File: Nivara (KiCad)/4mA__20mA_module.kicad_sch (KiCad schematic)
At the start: 2 parts

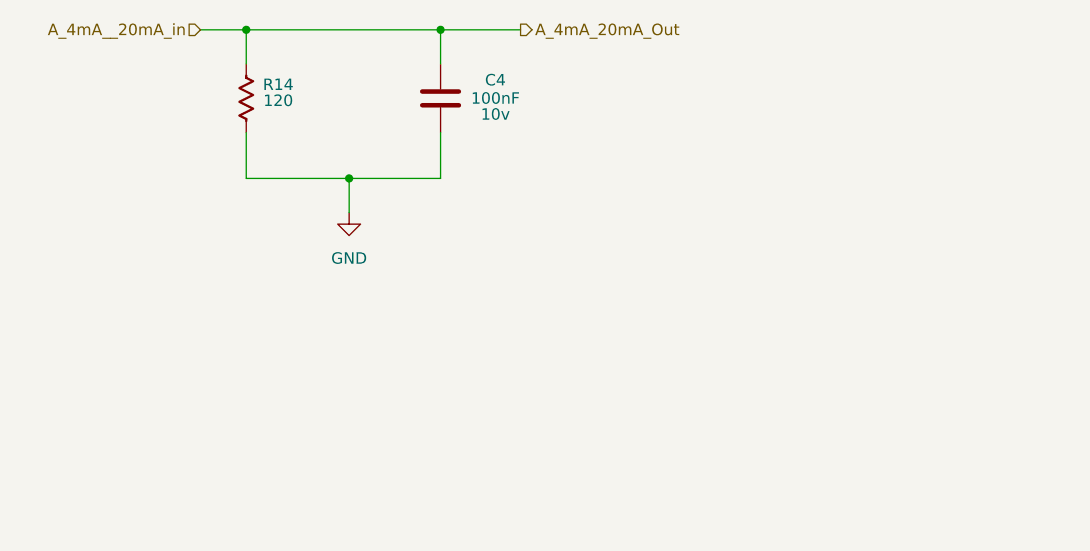
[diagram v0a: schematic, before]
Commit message: Add files via upload
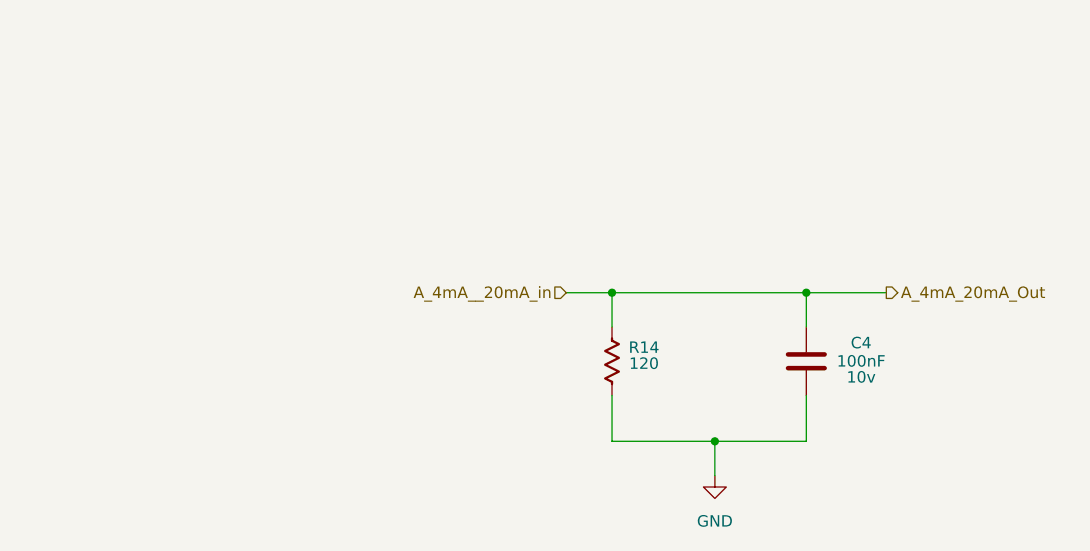
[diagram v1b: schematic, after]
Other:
- moved on the sheet: C4, R14
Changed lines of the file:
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@@
 	(paper "A4")
 	(junction
-		(at 100.33 86.36)
+		(at 140.97 115.57)
 		(diameter 0)
 		(color 0 0 0 0)
 	)
 	(junction
-		(at 110.49 69.85)
+		(at 151.13 99.06)
 		(diameter 0)
 		(color 0 0 0 0)
 	)
 	(junction
-		(at 88.9 69.85)
+		(at 129.54 99.06)
 		(diameter 0)
 		(color 0 0 0 0)
@@
 	(wire
 		(pts
-			(xy 88.9 81.28) (xy 88.9 86.36)
-		)
-		(stroke
-			(width 0)
-			(type default)
-		)
-	)
-	(wire
-		(pts
-			(xy 110.49 81.28) (xy 110.49 86.36)
-		)
-		(stroke
-			(width 0)
-			(type default)
-		)
-	)
-	(wire
-		(pts
-			(xy 110.49 69.85) (xy 88.9 69.85)
-		)
-		(stroke
-			(width 0)
-			(type default)
-		)
-	)
-	(wire
-		(pts
-			(xy 100.33 86.36) (xy 110.49 86.36)
-		)
-		(stroke
-			(width 0)
-			(type default)
-		)
-	)
-	(wire
-		(pts
-			(xy 88.9 73.66) (xy 88.9 69.85)
-		)
-		(stroke
-			(width 0)
-			(type default)
-		)
-	)
-	(wire
-		(pts
-			(xy 88.9 69.85) (xy 83.82 69.85)
-		)
-		(stroke
-			(width 0)
-			(type default)
-		)
-	)
-	(wire
-		(pts
-			(xy 100.33 86.36) (xy 100.33 90.17)
-		)
-		(stroke
-			(width 0)
-			(type default)
-		)
-	)
-	(wire
-		(pts
-			(xy 88.9 86.36) (xy 100.33 86.36)
-		)
-		(stroke
-			(width 0)
-			(type default)
-		)
-	)
-	(wire
-		(pts
-			(xy 110.49 69.85) (xy 110.49 73.66)
-		)
-		(stroke
-			(width 0)
-			(type default)
-		)
-	)
-	(wire
-		(pts
-			(xy 110.49 69.85) (xy 119.38 69.85)
+			(xy 129.54 110.49) (xy 129.54 115.57)
+		)
+		(stroke
+			(width 0)
+			(type default)
+		)
+	)
+	(wire
+		(pts
+			(xy 151.13 110.49) (xy 151.13 115.57)
+		)
+		(stroke
+			(width 0)
+			(type default)
+		)
+	)
+	(wire
+		(pts
+			(xy 151.13 99.06) (xy 129.54 99.06)
+		)
+		(stroke
+			(width 0)
+			(type default)
+		)
+	)
+	(wire
+		(pts
+			(xy 140.97 115.57) (xy 151.13 115.57)
+		)
+		(stroke
+			(width 0)
+			(type default)
+		)
+	)
+	(wire
+		(pts
+			(xy 129.54 102.87) (xy 129.54 99.06)
+		)
+		(stroke
+			(width 0)
+			(type default)
+		)
+	)
+	(wire
+		(pts
+			(xy 129.54 99.06) (xy 124.46 99.06)
+		)
+		(stroke
+			(width 0)
+			(type default)
+		)
+	)
+	(wire
+		(pts
+			(xy 140.97 115.57) (xy 140.97 119.38)
+		)
+		(stroke
+			(width 0)
+			(type default)
+		)
+	)
+	(wire
+		(pts
+			(xy 129.54 115.57) (xy 140.97 115.57)
+		)
+		(stroke
+			(width 0)
+			(type default)
+		)
+	)
+	(wire
+		(pts
+			(xy 151.13 99.06) (xy 151.13 102.87)
+		)
+		(stroke
+			(width 0)
+			(type default)
+		)
+	)
+	(wire
+		(pts
+			(xy 151.13 99.06) (xy 160.02 99.06)
 		)
 		(stroke
@@
 	(hierarchical_label "A_4mA__20mA_in"
 		(shape input)
-		(at 83.82 69.85 180)
+		(at 124.46 99.06 180)
 		(effects
 			(font
@@
 	(hierarchical_label "A_4mA_20mA_Out"
 		(shape output)
-		(at 119.38 69.85 0)
+		(at 160.02 99.06 0)
 		(effects
 			(font
@@
 	(symbol
 		(lib_id "PCM_Capacitor_US_AKL:C_0603")
-		(at 110.49 77.47 180)
+		(at 151.13 106.68 180)
 		(unit 1)
 		(exclude_from_sim no)
@@
 		(dnp no)
 		(property "Reference" "C4"
-			(at 116.586 75.438 0)
+			(at 157.226 104.648 0)
 			(effects
 				(font
@@
 		)
 		(property "Value" "C_0603"
-			(at 116.84 77.216 90)
+			(at 157.48 106.426 90)
 			(effects
 				(font
@@
 		)
 		(property "Footprint" "PCM_Capacitor_SMD_AKL:C_0603_1608Metric"
-			(at 109.5248 73.66 0)
+			(at 150.1648 102.87 0)
 			(effects
 				(font
@@
 		)
 		(property "Datasheet" "~"
-			(at 110.49 77.47 0)
+			(at 151.13 106.68 0)
 			(effects
 				(font
@@
 		)
 		(property "Description" "SMD 0603 MLCC capacitor, Alternate KiCad Library"
-			(at 110.49 77.47 0)
+			(at 151.13 106.68 0)
 			(effects
 				(font
@@
 		)
 		(property "Capacidad" "100nF"
-			(at 116.586 77.47 0)
+			(at 157.226 106.68 0)
 			(effects
 				(font
@@
 		)
 		(property "Part Number" ""
-			(at 110.49 77.47 0)
+			(at 151.13 106.68 0)
 			(effects
 				(font
@@
 		)
 		(property "Voltaje" "10v"
-			(at 116.586 79.248 0)
+			(at 157.226 108.458 0)
 			(effects
 				(font
@@
 	(symbol
 		(lib_id "power:GND")
-		(at 100.33 90.17 0)
+		(at 140.97 119.38 0)
 		(unit 1)
 		(exclude_from_sim no)
@@
 		(fields_autoplaced yes)
 		(property "Reference" "#PWR033"
-			(at 100.33 96.52 0)
+			(at 140.97 125.73 0)
 			(effects
 				(font
@@
 		)
 		(property "Value" "GND"
-			(at 100.33 95.25 0)
+			(at 140.97 124.46 0)
 			(effects
 				(font
@@
 		)
 		(property "Footprint" ""
-			(at 100.33 90.17 0)
+			(at 140.97 119.38 0)
 			(effects
 				(font
@@
 		)
 		(property "Datasheet" ""
-			(at 100.33 90.17 0)
+			(at 140.97 119.38 0)
 			(effects
 				(font
@@
 		)
 		(property "Description" "Power symbol creates a global label with name \"GND\" , ground"
-			(at 100.33 90.17 0)
+			(at 140.97 119.38 0)
 			(effects
 				(font
@@
 	(symbol
 		(lib_id "PCM_Resistor_US_AKL:R_0603")
-		(at 88.9 77.47 0)
+		(at 129.54 106.68 0)
 		(unit 1)
 		(exclude_from_sim no)
@@
 		(dnp no)
 		(property "Reference" "R14"
-			(at 92.456 75.946 0)
+			(at 133.096 105.156 0)
 			(effects
 				(font
@@
 		)
 		(property "Value" "R_0603"
-			(at 81.534 77.47 90)
+			(at 122.174 106.68 90)
 			(effects
 				(font
@@
 		)
 		(property "Footprint" "PCM_Resistor_SMD_AKL:R_0603_1608Metric"
-			(at 88.9 88.9 0)
+			(at 129.54 118.11 0)
 			(effects
 				(font
@@
 		)
 		(property "Datasheet" "~"
-			(at 88.9 77.47 0)
+			(at 129.54 106.68 0)
 			(effects
 				(font
@@
 		)
 		(property "Description" "SMD 0603 Chip Resistor, US Symbol, Alternate KiCad Library"
-			(at 88.9 77.47 0)
+			(at 129.54 106.68 0)
 			(effects
 				(font
@@
 		)
 		(property "Part Number" ""
-			(at 88.9 77.47 0)
+			(at 129.54 106.68 0)
 			(effects
 				(font
@@
 		)
 		(property "Capacidad" "120"
-			(at 92.456 77.724 0)
-			(effects
-				(font
+			(at 133.096 106.934 0)
+			(effects
+				(font
